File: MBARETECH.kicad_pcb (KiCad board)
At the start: 2 copper layers, 100 x 104 mm, 6 parts

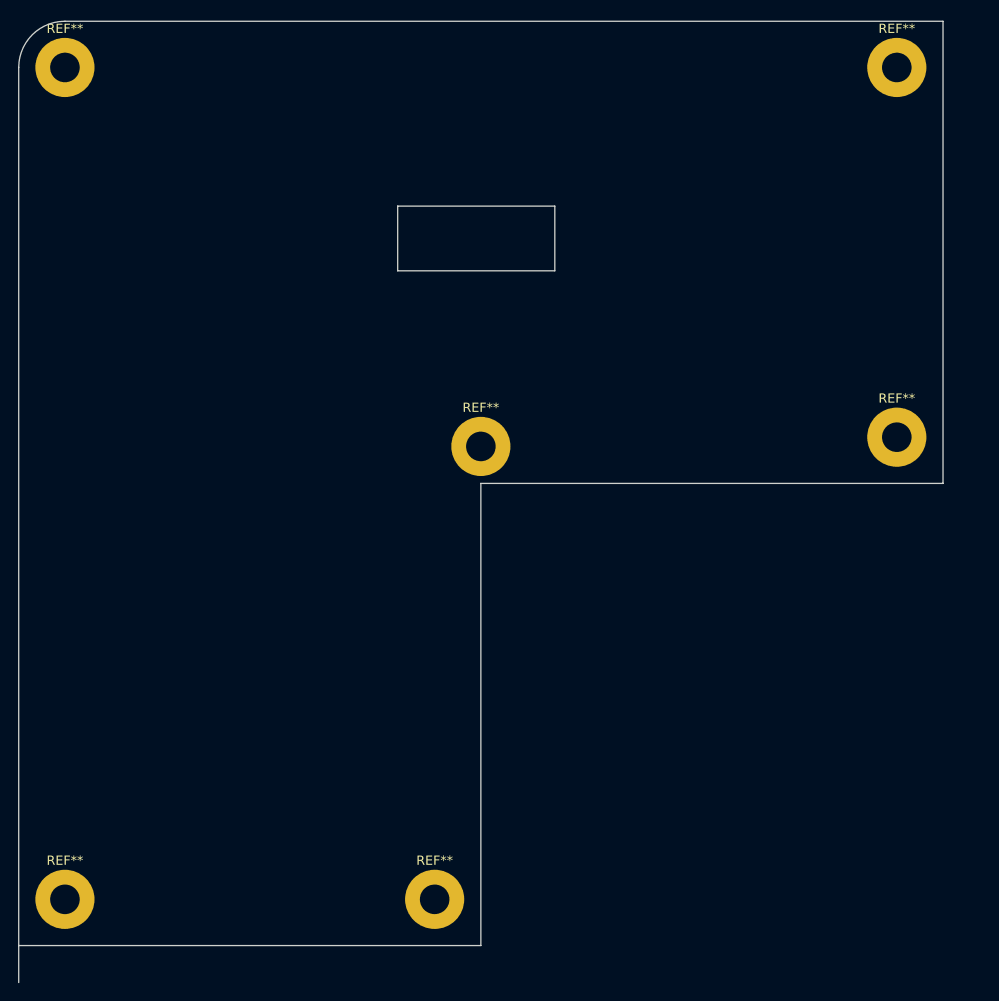
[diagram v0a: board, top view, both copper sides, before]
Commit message: Version final
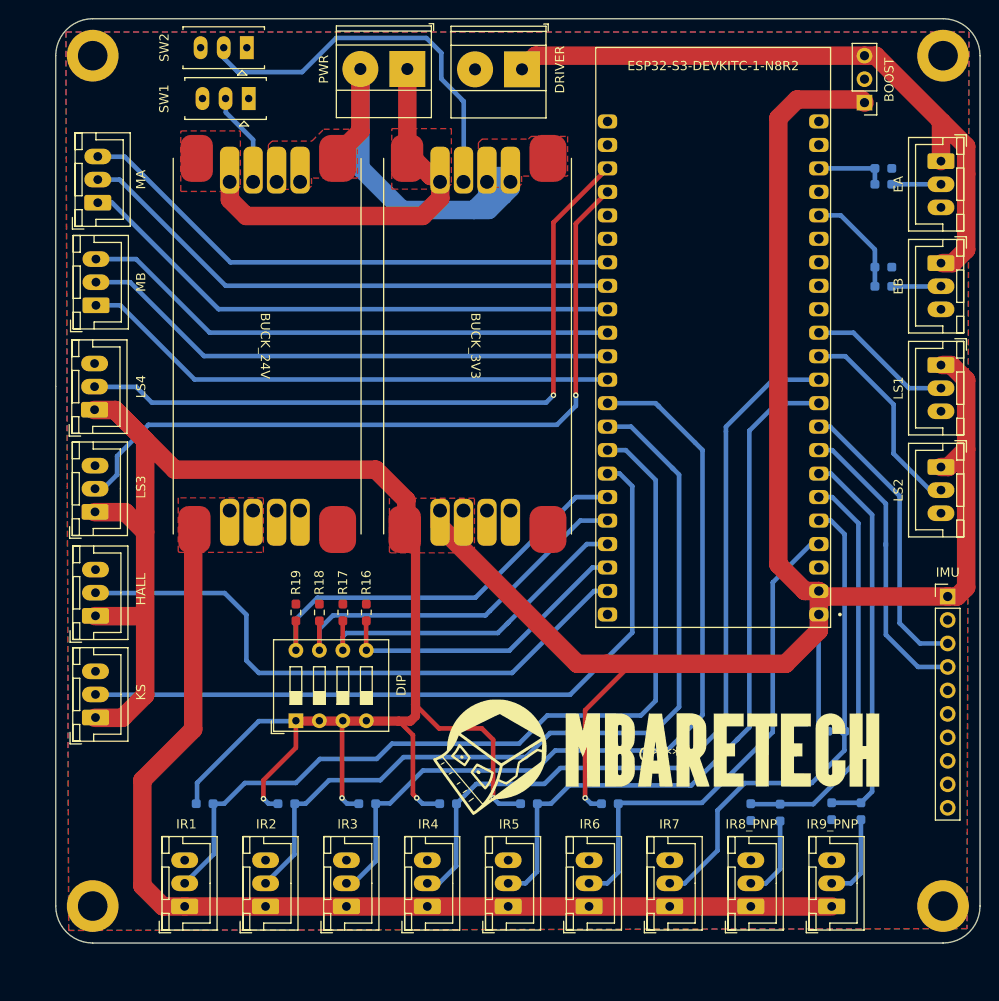
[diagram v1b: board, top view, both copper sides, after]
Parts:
- removed REF** (x6): MountingHole_3.2mm_M3_Pad, MountingHole:MountingHole_3.2mm_M3_Pad
- added ?: , , F.Cu at (193.2, 56.2)
- added ?: , , F.Cu at (101.0, 149.7)
- added ?: , , F.Cu at (101.0, 56.2)
- added ?: , , F.Cu at (193.0, 148.7)
- added BUCK1: BUCK_24V, Mbaretech_buckConverter:Buck-Converter, F.Cu at (109.7, 67.8)
- added BUCK2: BUCK_3V3, Mbaretech_buckConverter:Buck-Converter, F.Cu at (132.5, 67.8)
- added Boost1: BOOST, Connector_PinHeader_2.54mm:PinHeader_1x03_P2.54mm_Vertical, F.Cu at (184.5, 61.8)
- added DIP1: DIP, Button_Switch_THT:SW_DIP_SPSTx04_Slide_9.78x12.34mm_W7.62mm_P2.54mm, F.Cu at (123.0, 128.7)
- added DRIVER1: DRIVER, TerminalBlock_Phoenix:TerminalBlock_Phoenix_MKDS-1,5-2-5.08_1x02_P5.08mm_Horizontal, F.Cu at (147.4, 58.2)
- added EA1: EA, Connector_JST:JST_XH_B3B-XH-A_1x03_P2.50mm_Vertical, F.Cu at (192.8, 68.1)
- added EB1: EB, Connector_JST:JST_XH_B3B-XH-A_1x03_P2.50mm_Vertical, F.Cu at (192.8, 79.2)
- added G***: LOGO, Mbaretech_buckConverter:mbaretech_logo_fp, F.Cu at (162.4, 132.3)
- added HALL1: HALL, Connector_JST:JST_XH_B3B-XH-A_1x03_P2.50mm_Vertical, F.Cu at (101.3, 117.3)
- added IMU1: IMU, Connector_PinHeader_2.54mm:PinHeader_1x10_P2.54mm_Vertical, F.Cu at (193.5, 115.2)
- added IR1: IR1, Connector_JST:JST_XH_B3B-XH-A_1x03_P2.50mm_Vertical, F.Cu at (111.0, 148.8)
- added IR2: IR2, Connector_JST:JST_XH_B3B-XH-A_1x03_P2.50mm_Vertical, F.Cu at (119.7, 148.8)
- added IR3: IR3, Connector_JST:JST_XH_B3B-XH-A_1x03_P2.50mm_Vertical, F.Cu at (128.5, 148.8)
- added IR4: IR4, Connector_JST:JST_XH_B3B-XH-A_1x03_P2.50mm_Vertical, F.Cu at (137.2, 148.8)
- added IR5: IR5, Connector_JST:JST_XH_B3B-XH-A_1x03_P2.50mm_Vertical, F.Cu at (146.0, 148.8)
- added IR6_NPN1: IR6, Connector_JST:JST_XH_B3B-XH-A_1x03_P2.50mm_Vertical, F.Cu at (154.7, 148.8)
- added IR7: IR7, Connector_JST:JST_XH_B3B-XH-A_1x03_P2.50mm_Vertical, F.Cu at (163.4, 148.8)
- added IR8: IR8_PNP, Connector_JST:JST_XH_B3B-XH-A_1x03_P2.50mm_Vertical, F.Cu at (172.2, 148.8)
- added IR9: IR9_PNP, Connector_JST:JST_XH_B3B-XH-A_1x03_P2.50mm_Vertical, F.Cu at (181.0, 148.8)
- added KS1: KS, Connector_JST:JST_XH_B3B-XH-A_1x03_P2.50mm_Vertical, F.Cu at (101.3, 128.3)
- added LS1: LS1, Connector_JST:JST_XH_B3B-XH-A_1x03_P2.50mm_Vertical, F.Cu at (192.8, 90.2)
- added LS2: LS2, Connector_JST:JST_XH_B3B-XH-A_1x03_P2.50mm_Vertical, F.Cu at (192.8, 101.2)
- added LS3: LS3, Connector_JST:JST_XH_B3B-XH-A_1x03_P2.50mm_Vertical, F.Cu at (101.3, 106.1)
- added LS4: LS4, Connector_JST:JST_XH_B3B-XH-A_1x03_P2.50mm_Vertical, F.Cu at (101.2, 95.0)
- added MA1: MA, Connector_JST:JST_XH_B3B-XH-A_1x03_P2.50mm_Vertical, F.Cu at (101.6, 72.6)
- added MB1: MB, Connector_JST:JST_XH_B3B-XH-A_1x03_P2.50mm_Vertical, F.Cu at (101.4, 83.7)
- added PWR1: PWR, TerminalBlock_Phoenix:TerminalBlock_Phoenix_MKDS-1,5-2-5.08_1x02_P5.08mm_Horizontal, F.Cu at (135.0, 58.2)
- added R1: R1, Resistor_SMD:R_0603_1608Metric_Pad0.98x0.95mm_HandSolder, B.Cu at (113.1, 137.7)
- added R10: R10, Resistor_SMD:R_0603_1608Metric_Pad0.98x0.95mm_HandSolder, B.Cu at (184.1, 138.5)
- added R11: R11, Resistor_SMD:R_0603_1608Metric_Pad0.98x0.95mm_HandSolder, B.Cu at (181.0, 138.5)
- added R12: R12, Resistor_SMD:R_0603_1608Metric_Pad0.98x0.95mm_HandSolder, B.Cu at (186.5, 70.6)
- added R13: R13, Resistor_SMD:R_0603_1608Metric_Pad0.98x0.95mm_HandSolder, B.Cu at (186.5, 68.9)
- added R14: R14, Resistor_SMD:R_0603_1608Metric_Pad0.98x0.95mm_HandSolder, B.Cu at (186.5, 81.7)
- added R15: R15, Resistor_SMD:R_0603_1608Metric_Pad0.98x0.95mm_HandSolder, B.Cu at (186.5, 79.6)
- added R16: R16, Resistor_SMD:R_0603_1608Metric_Pad0.98x0.95mm_HandSolder, F.Cu at (130.6, 117.0)
- added R17: R17, Resistor_SMD:R_0603_1608Metric_Pad0.98x0.95mm_HandSolder, F.Cu at (128.1, 117.0)
- added R18: R18, Resistor_SMD:R_0603_1608Metric_Pad0.98x0.95mm_HandSolder, F.Cu at (125.5, 117.0)
- added R19: R19, Resistor_SMD:R_0603_1608Metric_Pad0.98x0.95mm_HandSolder, F.Cu at (123.0, 117.0)
- added R2: R2, Resistor_SMD:R_0603_1608Metric_Pad0.98x0.95mm_HandSolder, B.Cu at (122.0, 137.7)
- added R3: R3, Resistor_SMD:R_0603_1608Metric_Pad0.98x0.95mm_HandSolder, B.Cu at (130.7, 137.7)
- added R4: R4, Resistor_SMD:R_0603_1608Metric_Pad0.98x0.95mm_HandSolder, B.Cu at (139.5, 137.7)
- added R5: R5, Resistor_SMD:R_0603_1608Metric_Pad0.98x0.95mm_HandSolder, B.Cu at (148.2, 137.7)
- added R6: R6, Resistor_SMD:R_0603_1608Metric_Pad0.98x0.95mm_HandSolder, B.Cu at (157.0, 137.7)
- added R7: R7, Resistor_SMD:R_0603_1608Metric_Pad0.98x0.95mm_HandSolder, B.Cu at (181.4, 129.8)
- added R8: R8, Resistor_SMD:R_0603_1608Metric_Pad0.98x0.95mm_HandSolder, B.Cu at (175.4, 138.6)
- added R9: R9, Resistor_SMD:R_0603_1608Metric_Pad0.98x0.95mm_HandSolder, B.Cu at (172.2, 138.6)
- added SW1: SW1, SPDT_SlideSwitch:tht, F.Cu at (117.4, 61.4)
- added SW2: SW2, SPDT_SlideSwitch:tht, F.Cu at (117.2, 55.9)
- added U1: ESP32-S3-DEVKITC-1-N8R2, ESP32-S3-DEVKITC-1-N8R2:XCVR_ESP32-S3-DEVKITC-1-N8R2, F.Cu at (168.1, 87.2)
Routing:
- net +3V3: track 0.00 -> 390.5 mm, vias 0 -> 5
- net +24V: track 0.00 -> 117.0 mm
- net IR1_3V3: track 0.00 -> 92.8 mm
- net IR2_3V3: track 0.00 -> 92.0 mm
- net IR3_3V3: track 0.00 -> 91.1 mm
- net IR4_3V3: track 0.00 -> 87.6 mm
- net LS3_3V3: track 0.00 -> 81.6 mm, vias 0 -> 1
- net KILLSWITCH: track 0.00 -> 80.0 mm
- net IR5_3V3: track 0.00 -> 78.5 mm
- net LS4_3V3: track 0.00 -> 77.8 mm, vias 0 -> 1
- net +5V: track 0.00 -> 71.5 mm
- net HALL_3V3: track 0.00 -> 65.6 mm
- net PWMA: track 0.00 -> 60.1 mm
- net A1: track 0.00 -> 60.0 mm
- net A0: track 0.00 -> 59.9 mm
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- added copper zone on F.Cu, net +24V
- added copper zone on F.Cu, net +3V3
- added copper zone on F.Cu, net +BATT
- added copper zone on F.Cu, net -BATT
- added copper zone on B.Cu, net GND
- added copper zone on F.Cu, net GND
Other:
- board size 100 x 104 mm -> 100 x 100 mm
